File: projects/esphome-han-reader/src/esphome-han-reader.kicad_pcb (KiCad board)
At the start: 2 copper layers, 45.5 x 52.2 mm, 16 parts, among them J1 RJ12, J2 ProgammingPins, Q1 BC817W, SW1 ResetBtn, SW2 FlashBtn, U1 ESP-07, U2 LD1117S33CTR_SOT223

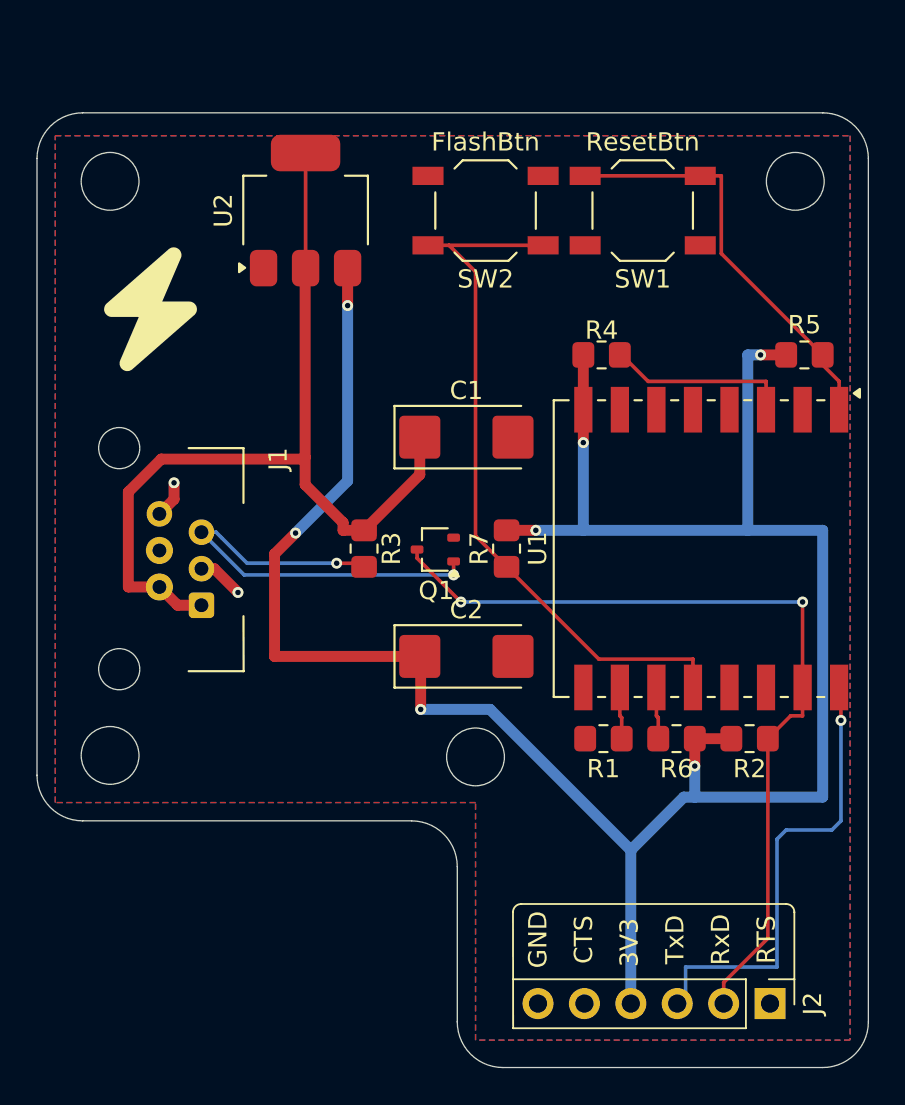
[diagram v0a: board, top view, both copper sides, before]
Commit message: feat: new 3d file and kicad files
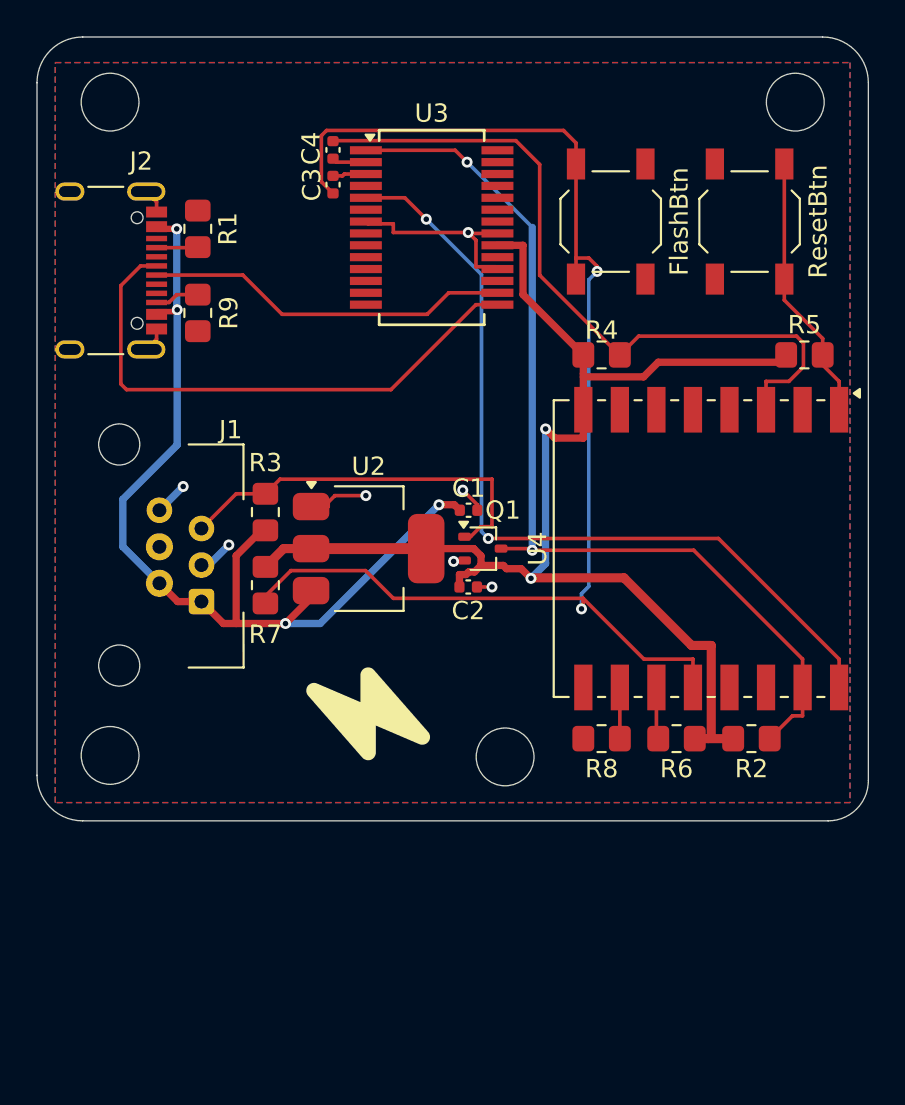
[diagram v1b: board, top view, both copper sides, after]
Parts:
- removed U1: ESP-07, RF_Module:ESP-07
- added C3: 0.1 µF, Capacitor_SMD:C_0402_1005Metric, F.Cu at (143.2, 77.2)
- added C4: 0.1 µF, Capacitor_SMD:C_0402_1005Metric, F.Cu at (143.2, 75.3)
- added R8: 10K, Resistor_SMD:R_0805_2012Metric_Pad1.20x1.40mm_HandSolder, F.Cu at (157.9, 107.5)
- added R9: 5K1, Resistor_SMD:R_0805_2012Metric_Pad1.20x1.40mm_HandSolder, F.Cu at (135.8, 84.2)
- added U3: FT232RL, Package_SO:SSOP-28_5.3x10.2mm_P0.65mm, F.Cu at (148.6, 79.5)
- added U4: ESP-07, RF_Module:ESP-07, F.Cu at (166.0, 97.1)
- C1: value 100nF -> 22uF; footprint Capacitor_Tantalum_SMD:CP_EIA-6032-15_Kemet-U_Pad2.25x2.35mm_HandSolder -> Capacitor_SMD:C_0402_1005Metric
- C2: value 10uF Polarized -> 22uF; footprint Capacitor_Tantalum_SMD:CP_EIA-6032-15_Kemet-U_Pad2.25x2.35mm_HandSolder -> Capacitor_SMD:C_0402_1005Metric
- J2: value ProgammingPins -> YTC-TC16-473; footprint Connector_PinHeader_2.54mm:PinHeader_1x06_P2.54mm_Vertical_NoSilkscreen -> Connector_USB:USB_C_Receptacle_XKB_U262-16XN-4BVC11
- R1: value 10K -> 5K1
- U2: value LD1117S33CTR_SOT223 -> TLV1117LV33DCYT
- moved J2 54.7 mm to (129.9, 81.9)
- moved R1 35.7 mm to (135.8, 79.6), turned to -90 degrees
- moved U2 18.8 mm to (145.2, 97.1), turned to 0 degrees
- moved R7 13.4 mm to (139.5, 99.1)
- moved SW2 6.88 mm to (158.4, 79.2), turned to 90 degrees
- moved SW1 5.88 mm to (166.0, 79.2), turned to 90 degrees
- moved R3 5.76 mm to (139.5, 95.1), turned to 90 degrees
- moved C1 4.00 mm to (150.6, 95.0), turned to 180 degrees
- moved C2 3.80 mm to (150.6, 99.2)
- moved Q1 2.60 mm to (151.4, 97.1), turned to 0 degrees
- moved J1 0.20 mm to (131.6, 97.1)
- moved R2 0.10 mm to (166.1, 107.5)
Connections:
- C1 pad 1: +5V -> GND
- C1 pad 2: GND -> +5V
- R1 pad 1: Net-(U1-GPIO15) -> GND
- R1 pad 2: GND -> USB-CC1
- U2 pad 2: +5V -> +3V3
- U2 pad 3: +3V3 -> +5V
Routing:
- net +3V3: track 127.1 -> 72.4 mm, vias 7 -> 2
- net GPIO 0: track 39.0 -> 74.2 mm, vias 0 -> 2
- net USB-DPOS: track 0.00 -> 30.4 mm
- net EN: track 10.1 -> 40.0 mm
- net ESP-TX: track 25.4 -> 46.2 mm, vias 1 -> 2
- net USB-DNEG: track 0.00 -> 20.0 mm
- net GND: track 4.75 -> 23.8 mm, vias 2 -> 7
- net RESET: track 22.9 -> 14.7 mm
- net ESP-RX: track 46.7 -> 53.0 mm
- net Net-(Q1-B): track 25.8 -> 21.3 mm, vias 2 -> 0
- net +5V: track 49.1 -> 53.2 mm, vias 0 -> 4
- net Net-(U1-GPIO15): track 2.84 -> 0.00 mm
- net Net-(U4-GPIO15): track 0.00 -> 2.80 mm
- net USB-CC2: track 0.00 -> 2.43 mm
- net USB-CC1: track 0.00 -> 2.27 mm
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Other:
- board size 45.5 x 52.2 mm -> 45.5 x 42.9 mm
- board text added: "GLÖM INTE SPARA"
- board text removed: "3V3"
- board text removed: "CTS"
- board text removed: "GND"
- board text removed: "RTS"
- board text removed: "RxD"
- board text removed: "TxD"
